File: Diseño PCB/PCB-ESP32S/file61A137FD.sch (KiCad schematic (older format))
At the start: 2 parts

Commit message: variables globales
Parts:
- TH?: symbol sensors:DHT22_Temperature_Humidity -> PCB-ESP32S-rescue:DHT22_Temperature_Humidity-sensors
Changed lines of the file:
@@
 $EndDescr
 $Comp
-L sensors:DHT22_Temperature_Humidity TH?
+L PCB-ESP32S-rescue:DHT22_Temperature_Humidity-sensors TH?
 U 1 1 61A00323
 P 2500 2350

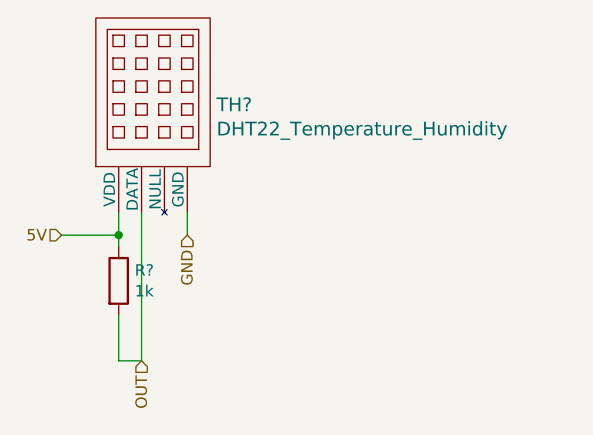
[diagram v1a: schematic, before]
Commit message: actualizando dibujo
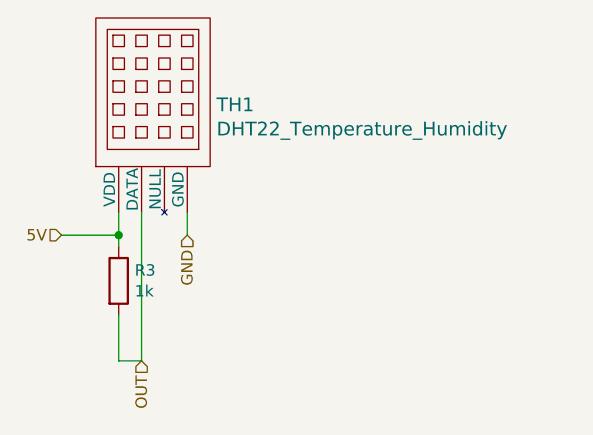
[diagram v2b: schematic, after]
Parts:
- gave numbers to parts that had none: 2
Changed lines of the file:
@@
 P 2500 2350
 AR Path="/61A00323" Ref="TH?"  Part="1"
-AR Path="/61A137FE/61A00323" Ref="TH?"  Part="1"
-F 0 "TH?" H 2778 2820 60  0000 L CNN
+AR Path="/61A137FE/61A00323" Ref="TH1"  Part="1"
+F 0 "TH1" H 2778 2820 60  0000 L CNN
 F 1 "DHT22_Temperature_Humidity" H 2778 2714 60  0000 L CNN
 F 2 "" H 2500 2350 60  0000 C CNN
@@
 P 2350 2650
 AR Path="/61A00339" Ref="R?"  Part="1"
-AR Path="/61A137FE/61A00339" Ref="R?"  Part="1"
-F 0 "R?" H 2420 2696 50  0000 L CNN
+AR Path="/61A137FE/61A00339" Ref="R3"  Part="1"
+F 0 "R3" H 2420 2696 50  0000 L CNN
 F 1 "1k" H 2420 2605 50  0000 L CNN
 F 2 "" V 2280 2650 50  0001 C CNN
